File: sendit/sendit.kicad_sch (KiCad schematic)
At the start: 1 part, among them U2 Seeed_Studio_XIAO_ESP32C6

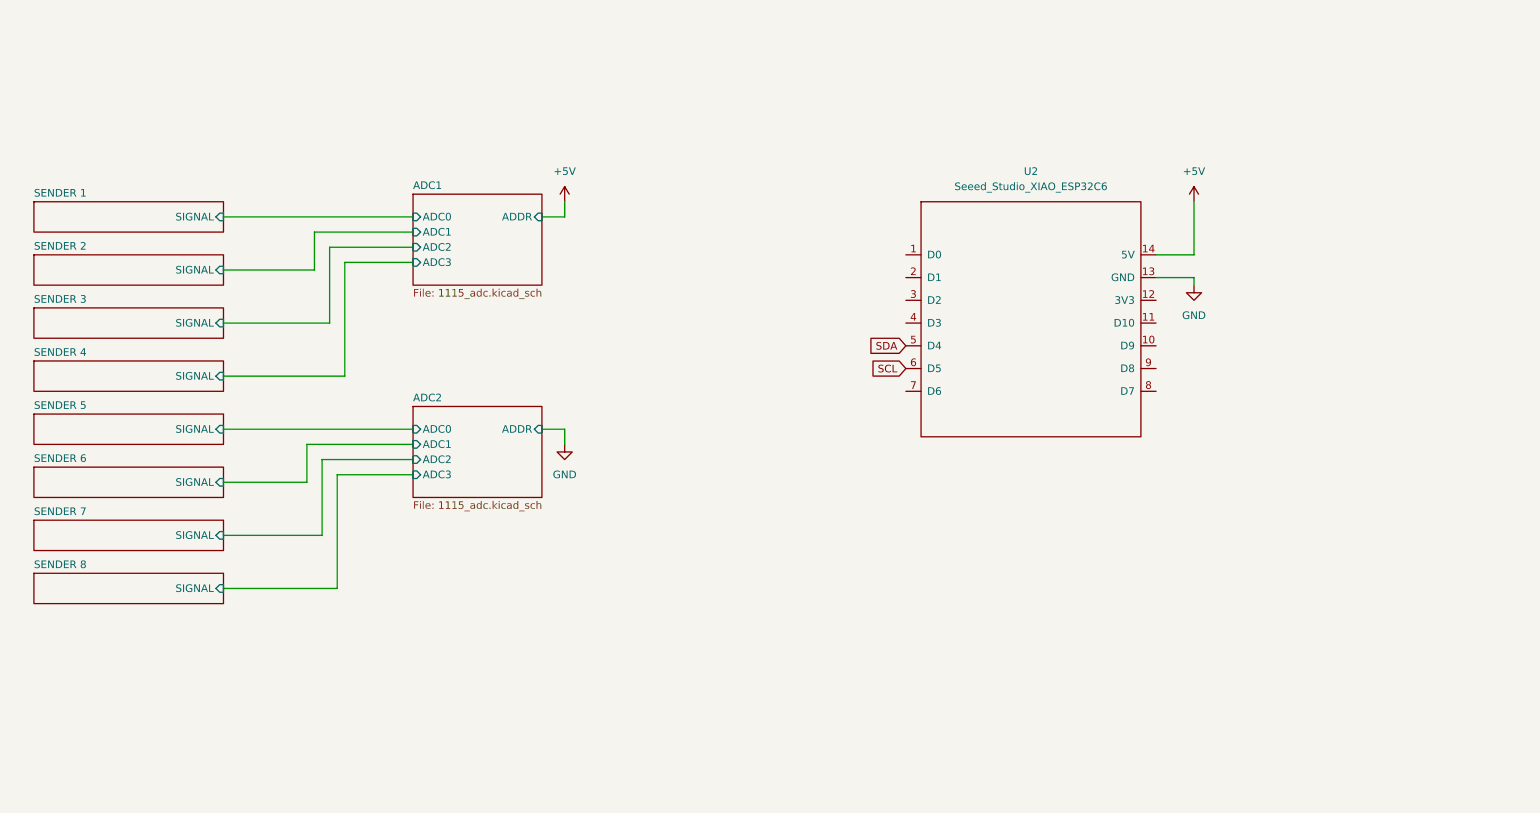
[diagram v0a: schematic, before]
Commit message: big update on the potential design.
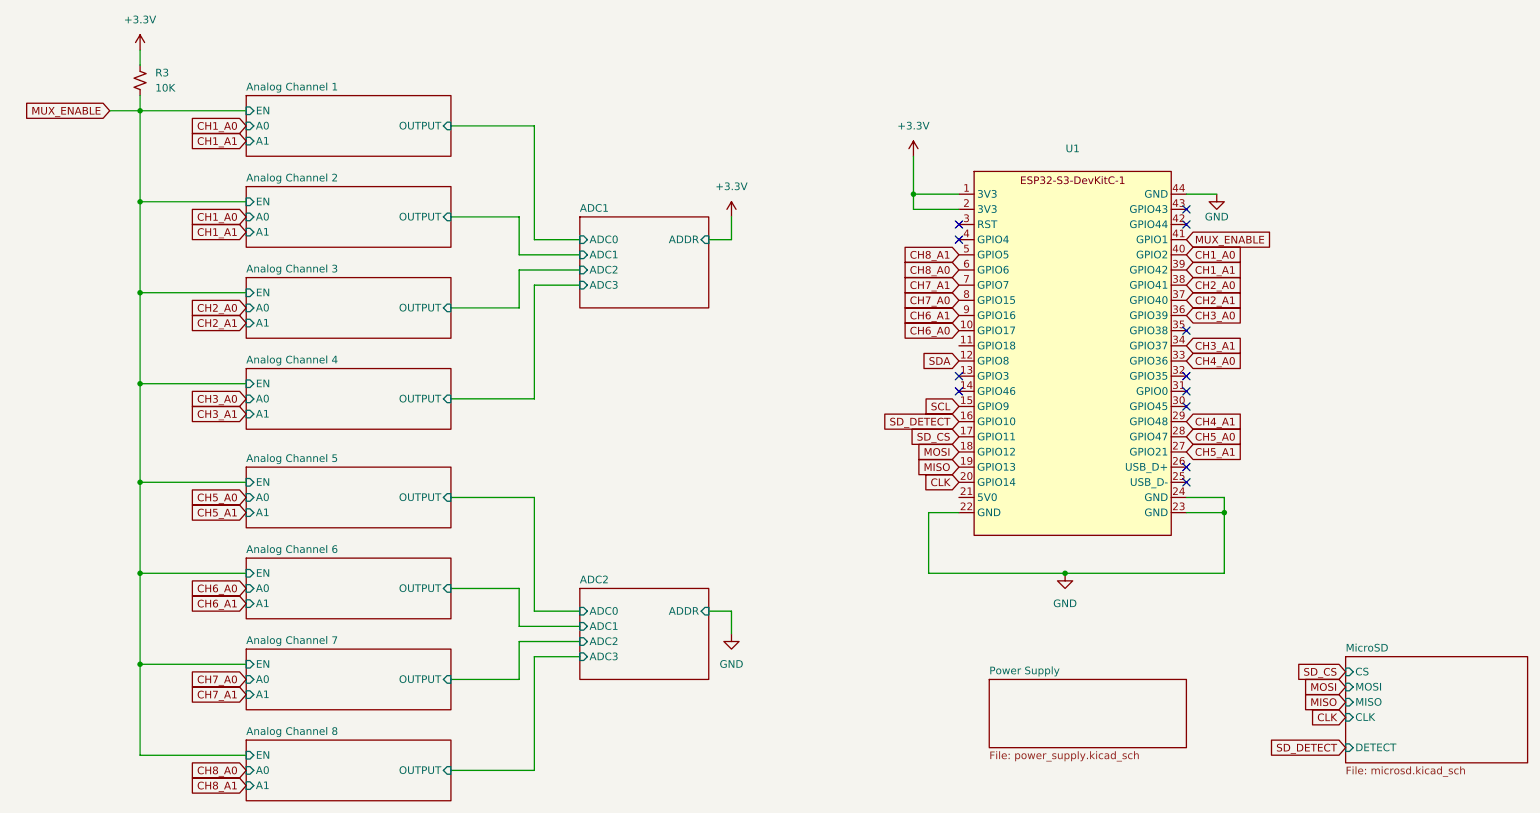
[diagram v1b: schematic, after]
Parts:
- removed U2: Seeed_Studio_XIAO_ESP32C6, Seeed Studio XIAO Series Library:XIAO-Generic-Hybrid-14P-2.54-21X17.8MM, symbol yarrboard:Seeed_Studio_XIAO_ESP32C6
- added R3: 10K, Resistor_SMD:R_1206_3216Metric_Pad1.30x1.75mm_HandSolder, symbol Device:R_Small_US
- added U1: ~, yarrboard:Waveshare-ESP32-S3-dev-kit-SMD, symbol yarrboard:ESP32-S3-DevKitC-1
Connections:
- net GND: now also U1.22 (GND), U1.23 (GND), U1.24 (GND), U1.44 (GND)
- net SCL: now also U1.15 (GPIO9)
- net SDA: now also U1.12 (GPIO8)
- new net +3.3V: R3.2, U1.1 (3V3), U1.2 (3V3)
- new net CH1_A0: U1.40 (GPIO2)
- new net CH1_A1: U1.39 (GPIO42)
- new net CH2_A0: U1.38 (GPIO41)
- new net CH2_A1: U1.37 (GPIO40)
- new net CH3_A0: U1.36 (GPIO39)
- new net CH3_A1: U1.34 (GPIO37)
- new net CH4_A0: U1.33 (GPIO36)
- new net CH4_A1: U1.29 (GPIO48)
- new net CH5_A0: U1.28 (GPIO47)
- new net CH5_A1: U1.27 (GPIO21)
- new net CH6_A0: U1.10 (GPIO17)
- new net CH6_A1: U1.9 (GPIO16)
- new net CH7_A0: U1.8 (GPIO15)
- new net CH7_A1: U1.7 (GPIO7)
- new net CH8_A0: U1.6 (GPIO6)
- new net CH8_A1: U1.5 (GPIO5)
- new net CLK: U1.20 (GPIO14)
- new net MISO: U1.19 (GPIO13)
- new net MOSI: U1.18 (GPIO12)
- new net MUX_ENABLE: R3.1, U1.41 (GPIO1)
- new net SD_CS: U1.17 (GPIO11)
- new net SD_DETECT: U1.16 (GPIO10)
- no-connect marks 0 -> 12
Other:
- removed sheet SENDER 1
- removed sheet SENDER 2
- removed sheet SENDER 3
- removed sheet SENDER 4
- removed sheet SENDER 5
- removed sheet SENDER 6
- removed sheet SENDER 7
- removed sheet SENDER 8
- added sheet Analog Channel 1 (analog_channel.kicad_sch)
- added sheet Analog Channel 2 (analog_channel.kicad_sch)
- added sheet Analog Channel 3 (analog_channel.kicad_sch)
- added sheet Analog Channel 4 (analog_channel.kicad_sch)
- added sheet Analog Channel 5 (analog_channel.kicad_sch)
- added sheet Analog Channel 6 (analog_channel.kicad_sch)
- added sheet Analog Channel 7 (analog_channel.kicad_sch)
- added sheet Analog Channel 8 (analog_channel.kicad_sch)
- added sheet MicroSD (microsd.kicad_sch)
- added sheet Power Supply (power_supply.kicad_sch)
